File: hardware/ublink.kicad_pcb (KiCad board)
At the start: 2 copper layers, 67 x 54.5 mm, 61 parts, among them J1 USB_B_Micro, J2 AC1, J3 5V Trafo, J4 Screw_Terminal_01x02, J5 Screw_Terminal_01x02, J7 Screw_Terminal_01x02, J8 Pin Header, J9 Screw_Terminal_01x02, Q1 STN3NF06L, Q2 RU6099, Q3 RU6099, Q4 RU6099, Q5 RU6099, Q6 STN3NF06L, SW1 SW_Push, SW2 SW_Push, SW3 JUC-31F, U1 3.3V3 Regul, U2 CH340G, U3 HF115F_005-1ZS3, U4 ESP32-WROOM-32U, U5 EL817S, U6 EL817S, U7 EL817S, U8 EL817S, Y1 12Mhz

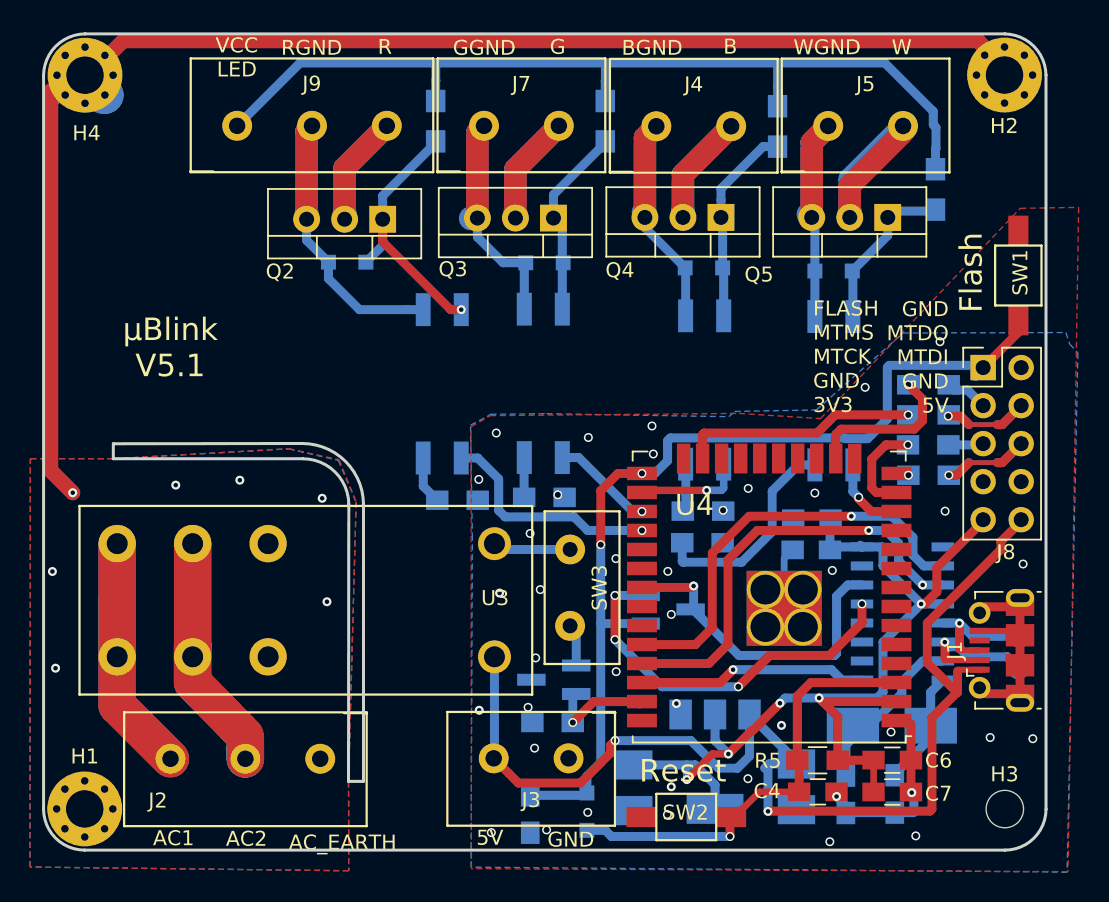
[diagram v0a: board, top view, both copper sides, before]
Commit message: stash
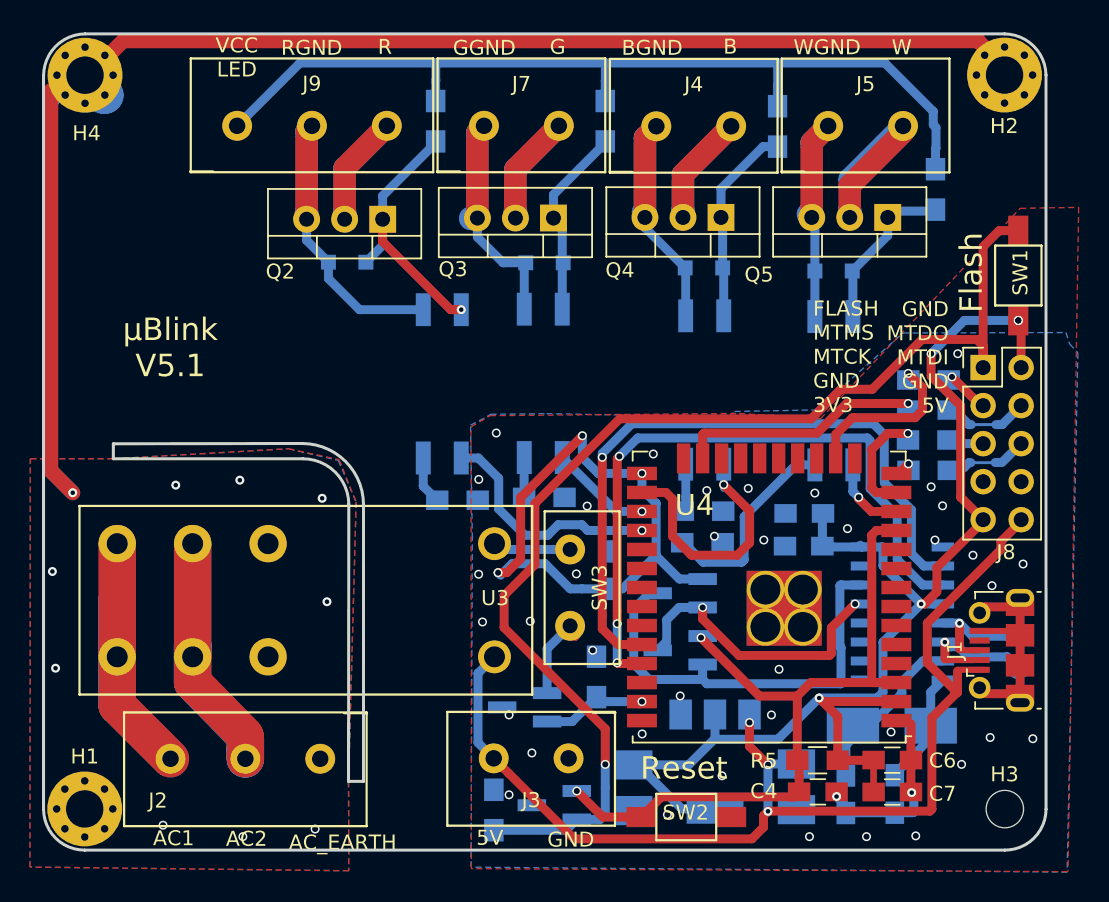
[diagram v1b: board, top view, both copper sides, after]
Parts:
- removed 2u2: CP2, Capacitors_SMD:C_0805_HandSoldering
- removed D5: D, Diodes_SMD:D_SOD-323_HandSoldering
- added C2: 2u, Capacitors_SMD:C_0805_HandSoldering, B.Cu at (148.1, 124.4)
- added Q7: STN3NF06L, TO_SOT_Packages_SMD:SOT-23_Handsoldering, B.Cu at (152.7, 129.8)
- added Q8: STN3NF06L, TO_SOT_Packages_SMD:SOT-23_Handsoldering, B.Cu at (152.7, 126.0)
- added R6: 10k, Resistors_SMD:R_0805_HandSoldering, B.Cu at (140.2, 140.5)
- moved Q6 15.1 mm to (144.2, 140.1), turned to 180 degrees
- moved R7 4.23 mm to (147.1, 131.6), turned to 90 degrees
- moved Q1 2.68 mm to (142.3, 133.6)
- moved 10u1 0.62 mm to (160.9, 120.7)
- moved C5 0.57 mm to (160.9, 122.8)
- moved R3 0.32 mm to (169.2, 111.7)
- moved R1 0.32 mm to (169.2, 115.7)
- moved R2 0.32 mm to (169.2, 117.8)
- moved R4 0.32 mm to (169.2, 113.7)
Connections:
- J8 pad 1: FLASH -> FLASH_BTN
- J8 pad 2: GND -> 3V3
- Q6 pad 1: FLASH -> EN
- Q6 pad 2: DTR -> FLASH_BTN
- Q6 pad 3: RTS -> GND
- SW1 pad 1: GND -> FLASH_BTN
- SW1 pad 2: FLASH -> 3V3
- SW2 pad 1: EN -> GND
- SW2 pad 2: GND -> EN
- U2 pad 9: CTS -> Net-(U2-Pad9)
- U4 pad 11: Net-(U4-Pad11) -> EN
- U4 pad 31: RTS -> Net-(U4-Pad31)
- U4 pad 36: CTS -> Net-(U4-Pad36)
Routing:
- net FLASH_BTN: track 0.00 -> 79.3 mm, vias 0 -> 1
- net FLASH: track 64.3 -> 40.2 mm, vias 2 -> 3
- net 3V3: track 68.5 -> 90.7 mm
- net EN: track 31.2 -> 52.1 mm, vias 1 -> 2
- net TX: track 29.6 -> 45.9 mm
- net RX: track 29.3 -> 45.3 mm, vias 2 -> 3
- net CTS: track 15.3 -> 0.00 mm, vias 1 -> 0
- net B_CTRL: track 7.89 -> 17.8 mm
- net RTS: track 21.8 -> 29.2 mm, vias 1 -> 0
- net DTR: track 25.8 -> 19.4 mm, vias 4 -> 2
- net Net-(J8-Pad6): track 10.7 -> 5.29 mm, vias 1 -> 0
- net Net-(J8-Pad4): track 10.5 -> 5.63 mm, vias 1 -> 0
- net GND: track 30.2 -> 26.1 mm
- net Net-(Q1-Pad1): track 2.82 -> 6.42 mm
- net 5V: track 78.0 -> 76.2 mm, vias 2 -> 3
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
